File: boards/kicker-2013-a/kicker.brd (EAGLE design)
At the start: 67 parts, among them J1 POWER, J2 CHIP, J3 KICK, J4 0528520870, Q1 STB40NF20, Q2 FGA180N33ATD-2, Q3 FGA180N33ATD-2, Q4 FDV303N, Q5 FQT1N80, T1 DA2034, U1 ADC081C027, U5 LT3757, U8 TC4427

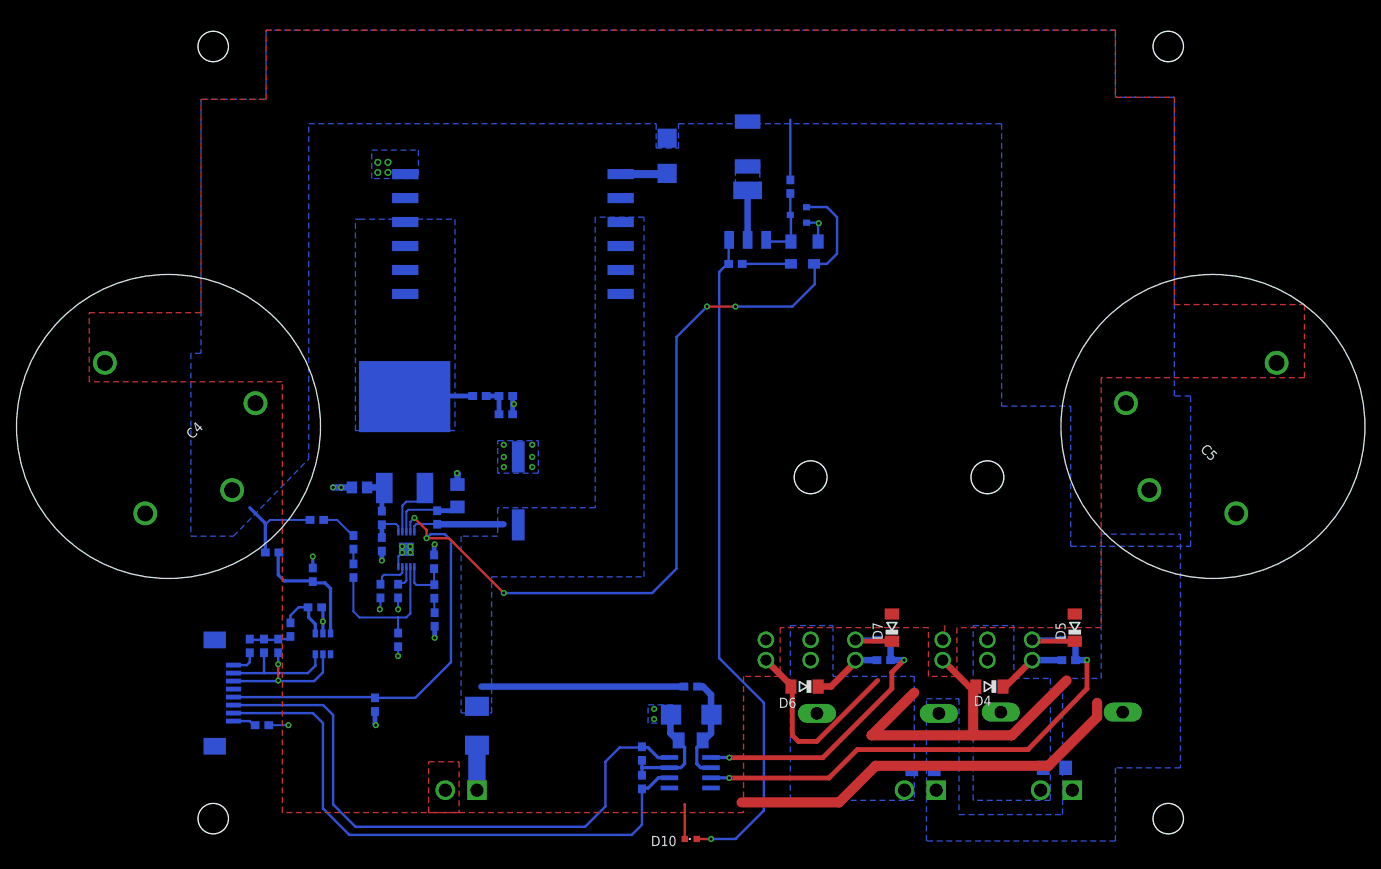
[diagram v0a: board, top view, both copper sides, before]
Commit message: kicker-2013-a
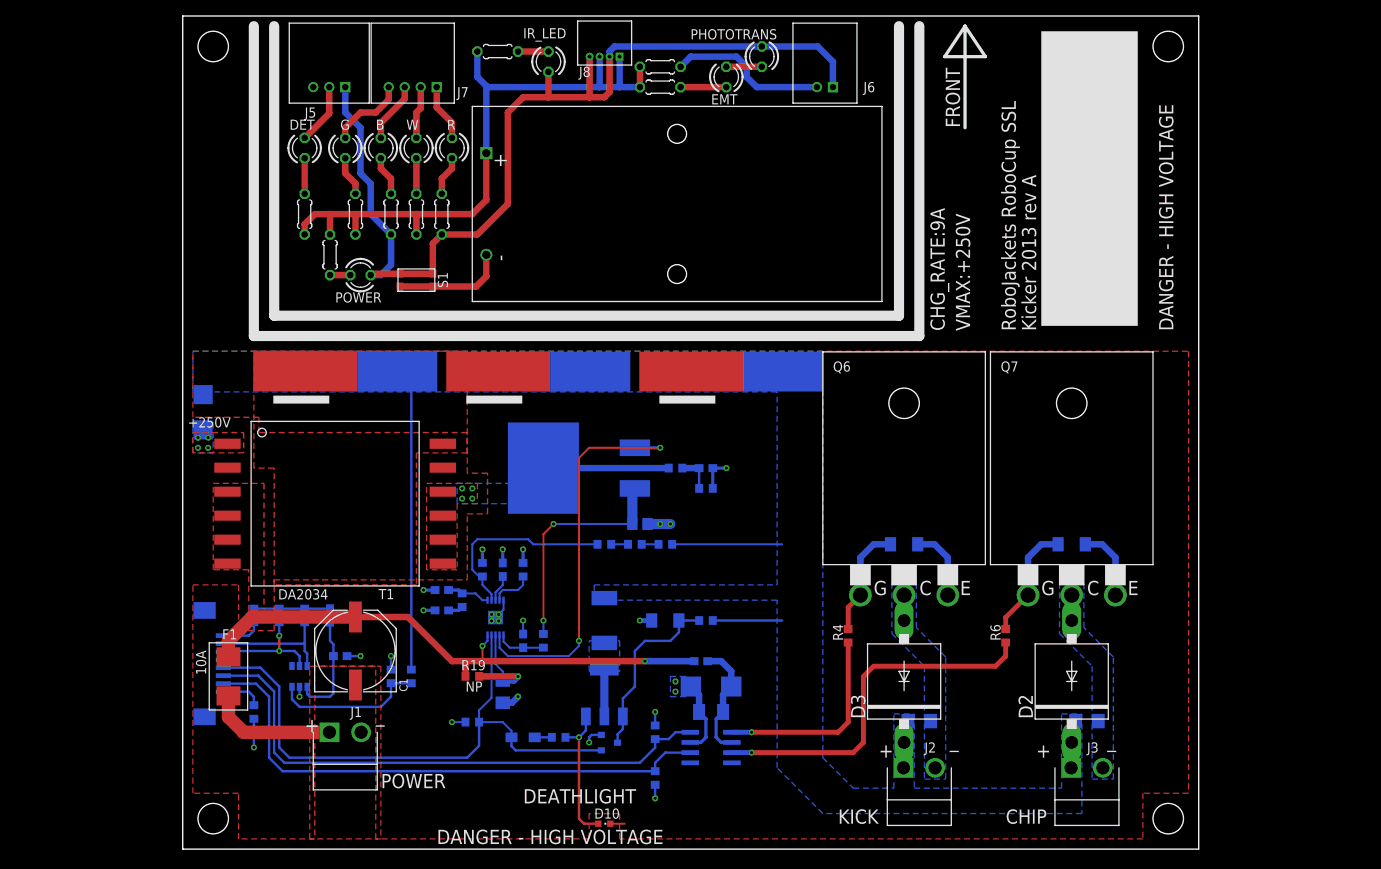
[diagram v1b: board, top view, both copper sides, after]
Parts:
- removed C4, C5: 2700uF 250V, panasonic:T-UP3
- removed D6, D7: BZV55-B18,115, diode:SOD80C
- removed Q2, Q3: FGA180N33ATD-2, fairchild:TOP3AH-2
- added B, DET, EMT, G, IR_LED, POWER, R, W: (no value), led:LED3MM
- added J5: 2MM-3H, 2mm:2MM-3-H
- added J6: 2MM-2H, 2mm:2MM-2-H
- added J7: 2MM-4H, 2mm:2MM-4-H
- added J8: 1.25MM-4H, 1.25mm:1.25MM-4-H
- added PHOTOTRANS: TLLG4400, led:LED3MM
- added Q6, Q7: IXGK400N30A3, IXYS:TO264
- added R30, R31, R32, R33, R35, R36, R37: (no value), resistor:0204/5
- added S1: KMR2, switch-robocup:KMR2
- added U$1: BATT-AAA-2, battholders:BATT-AAA-2
- added U$3, U$4, U$5: EET-UQ2E821CA, rc_caps:22CAP
- J2: value CHIP -> KICK
- J3: value KICK -> CHIP
- R3, R5: value 10 -> (none); device rcl:R0603 -> resistor:0204/5
- moved R3 104.1 mm to (14.6, 70.5), flipped to the top, turned to 90 degrees
- moved R5 84.8 mm to (17.8, 75.6), flipped to the top, turned to 270 degrees
- moved Q4 70.0 mm to (49.5, 9.53), turned to 270 degrees
- moved D9 68.7 mm to (38.7, 10.2), turned to 0 degrees
- moved D1 66.3 mm to (-1.27, 50.8)
- moved R29 63.2 mm to (43.2, 10.2), turned to 180 degrees
- moved Q5 62.2 mm to (48.9, 15.9)
- moved R27 62.2 mm to (48.9, 24.8)
- moved R28 55.2 mm to (61.6, 24.8), turned to 180 degrees
- moved D8 50.5 mm to (56.5, 24.8), turned to 0 degrees
- moved R21 43.7 mm to (56.5, 34.3), turned to 180 degrees
- moved T1 40.4 mm to (15.2, 39.4), flipped to the top
- moved R17 35.3 mm to (53.3, 36.8), turned to 0 degrees
- moved R22 35.2 mm to (52.7, 34.3), turned to 180 degrees
- moved F1 31.7 mm to (1.91, 17.8), flipped to the top
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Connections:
- removed net N$13: D2.A, J3.2, Q3.2A, Q3.2B, R16.1
- removed net N$19 (its old number): D7.C, Q3.1A, R5.2
- new net GND1: S1.1, S1.3, U$1.GND
- new net GND2: IR_LED.K, J5.1, J6.1, J8.2, J8.4, PHOTOTRANS.A, POWER.K, R30.2, R32.2, S1.2, S1.4
- new net N$1: D5.C, Q7.G, R6.2
- new net N$10: DET.A, R36.1
- new net N$18: DET.K, J5.2
- new net N$26: EMT.K, PHOTOTRANS.K
- new net N$34: G.A, R5.1
- new net N$35: B.K, R30.1
- new net N$36: R31.1, W.A
- new net N$38: R.K, R32.1
- new net N$39: EMT.A, R35.1
- new net N$42: J6.2, R37.1
- new net N$43: G.K, J7.4
- new net N$44: B.A, J7.3
- new net N$45: J7.2, W.K
- new net N$46: J7.1, R.A
- new net N$6: POWER.A, R3.1
- new net V+: J8.1, J8.3, R3.2, R31.2, R33.2, R35.2, R36.2, R37.2, R5.2, U$1.V+
- net GND: now also Q6.E, Q7.E, U$3.2, U$4.2, U$5.2; no longer C4.-, C5.-, D6.A, D7.A, Q2.3A, Q2.3B, Q3.3A, Q3.3B
- net HV: now also U$3.1, U$4.1, U$5.1; no longer C4.+, C5.+
- net N$11: now also D2.A, J3.2, Q7.C, R16.1; no longer D5.C, Q2.1A, R3.2
- net N$12: now also IR_LED.A, R33.1; no longer D6.C, Q3.1B, R6.2
- net N$15: now also U8.5; no longer R3.1, U8.7
- net N$16: now also U8.7; no longer R5.1, U8.5
- net N$17: now also Q6.C; no longer Q2.2A, Q2.2B
- net N$8: now also Q6.G; no longer Q2.1B
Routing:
- net GND2: track 0.00 -> 121.5 mm
- net GND: track 173.5 -> 68.3 mm, vias 31 -> 25
- net V+: track 0.00 -> 81.2 mm
- net CHARGE: track 152.4 -> 74.1 mm, vias 5 -> 0
- net N$30: track 84.1 -> 17.5 mm
- net N$2: track 8.15 -> 49.8 mm, vias 0 -> 2
- net HV: track 20.0 -> 57.1 mm
- net N$15: track 59.4 -> 25.0 mm, vias 2 -> 1
- net +12V: track 37.8 -> 69.3 mm, vias 0 -> 2
- net NAG: track 5.21 -> 28.7 mm, vias 0 -> 2
- net N$42: track 0.00 -> 19.9 mm
- net N$1: track 0.00 -> 14.5 mm
- net GND1: track 0.00 -> 14.0 mm
- net N$21: track 9.38 -> 22.8 mm
- net N$47: track 2.71 -> 15.7 mm, vias 0 -> 4
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- added copper zone on layer 1, net +12V
- added copper zone on layer 16, net N$11
- added copper zone on layer 1, net N$47
- added copper zone on layer 1, net N$50
- added copper zone on layer 16, net N$50
- removed copper zone on layer 16, net +12V
- removed copper zone on layer 16, net N$13
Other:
- board outline added: 127 x 104.1 mm
- board text added: "+250V"
- board text added: "ADC"
- board text added: "C"
- board text added: "CHG"
- board text added: "CHG_RATE:9A"
- board text added: "CHP"
- board text added: "DEATHLIGHT"
- board text added: "E"
- board text added: "Encoder Wire Tester"
- board text added: "FRONT"
- board text added: "G"
- board text added: "IR LED/Phototransistor Tester"
- board text added: "KCK"
- board text added: "Kicker 2013 rev A"
- board text added: "NP"
- board text added: "SCL"
- board text added: "SDA"
- board text added: "VMAX:+250V"
- board text added: "Version 1.1"
- board text added: "_"
- board text removed: "-"
- board text removed: "FROM CONTROL BOARD"
- board text removed: "Kicker 2011 rev C"
